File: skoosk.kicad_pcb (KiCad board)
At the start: 2 copper layers, 281.4 x 78.4 mm, 92 parts, among them SW1 SW_Push, U1 ProMicro

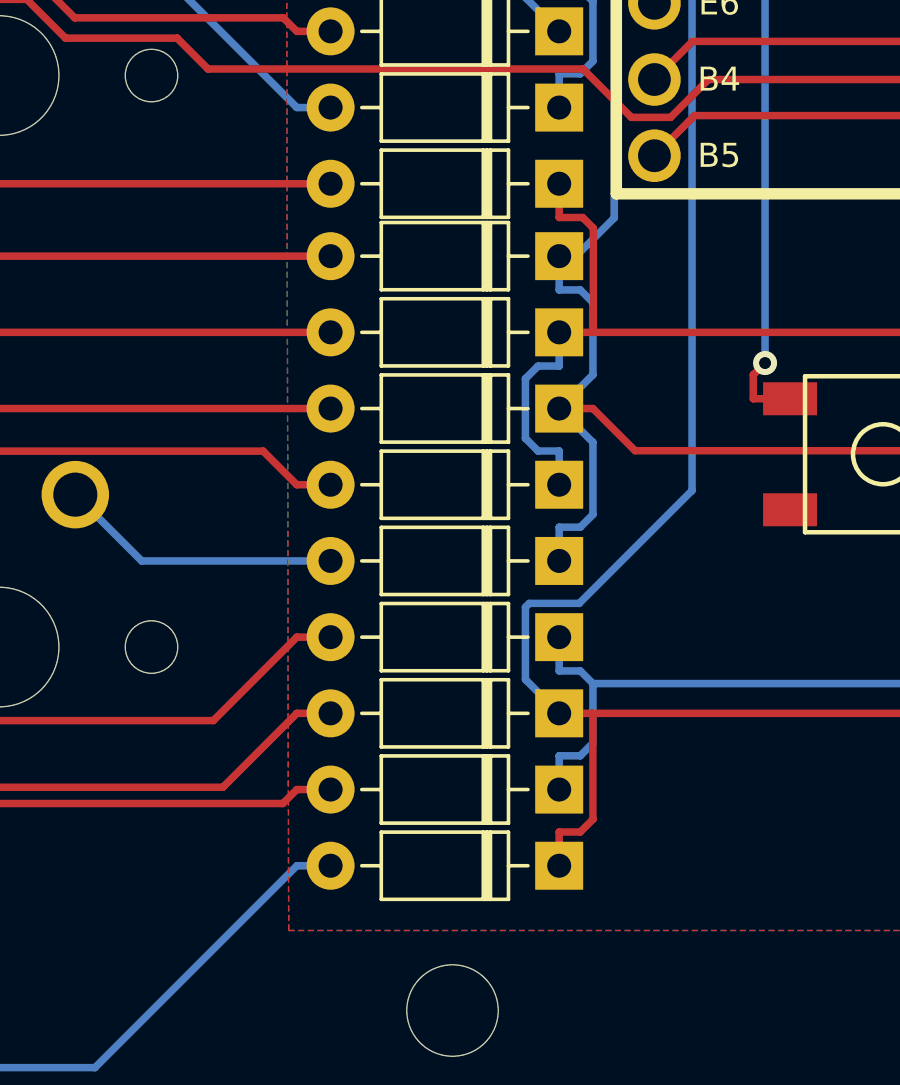
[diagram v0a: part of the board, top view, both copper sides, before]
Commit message: zero error return
add some led?
get feedback?
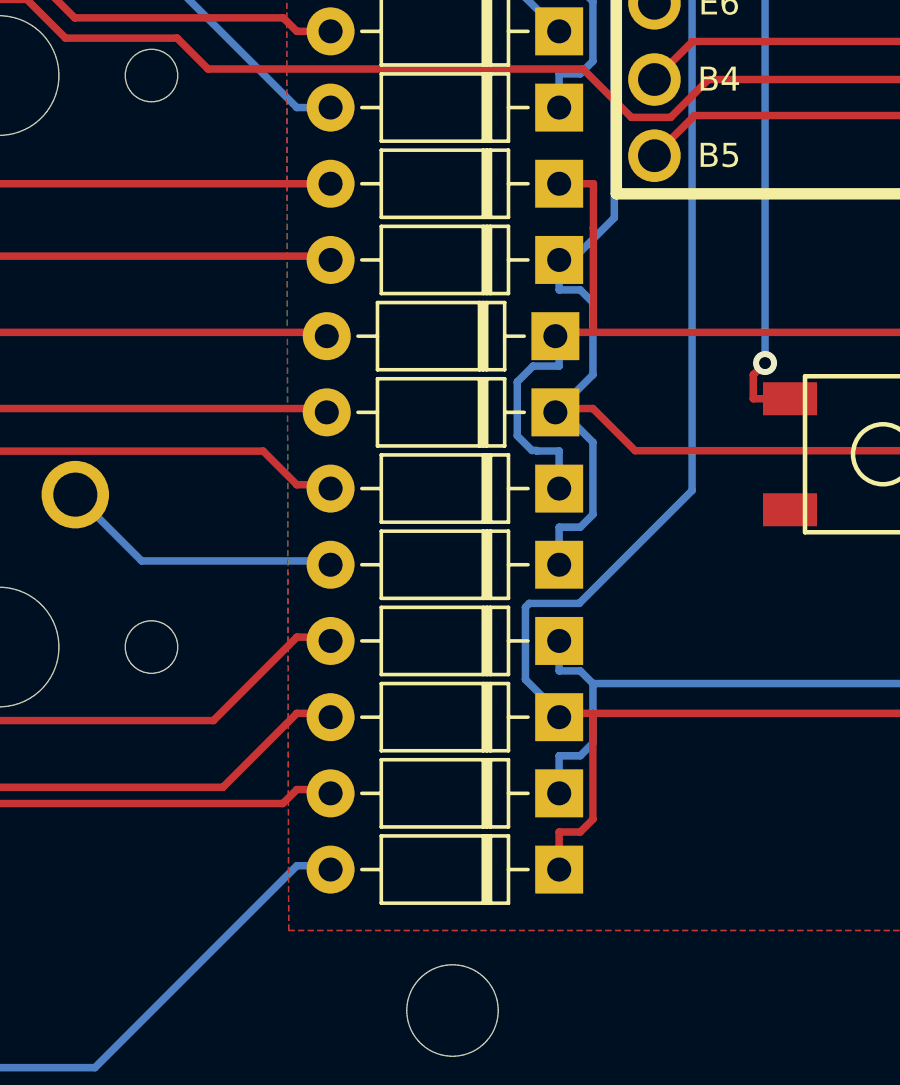
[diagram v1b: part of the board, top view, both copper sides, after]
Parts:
- moved D27 0.18 mm to (128.1, 49.1)
- moved D28 0.18 mm to (128.1, 51.7)
- moved D26 0.13 mm to (128.3, 46.6)
- moved D29 0.13 mm to (128.3, 54.2)
- moved D30 0.13 mm to (128.3, 56.8)
- moved D37 0.13 mm to (128.3, 59.3)
- moved D38 0.13 mm to (128.3, 61.8)
- moved D39 0.13 mm to (128.3, 64.4)
- moved D40 0.13 mm to (128.3, 66.9)
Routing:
- net ROW4: track 61.5 -> 62.1 mm
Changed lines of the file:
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@@
   (net 66 "unconnected-(U1-Pad1)")
   (footprint "Diode_THT:D_DO-35_SOD27_P7.62mm_Horizontal" (layer "F.Cu")
-    (at 128.27 51.562 180)
+    (at 128.143 51.689 180)
     (descr "Diode, DO-35_SOD27 series, Axial, Horizontal, pin pitch=7.62mm, , length*diameter=4*2mm^2, , http://www.diodes.com/_files/packages/DO-35.pdf")
     (tags "Diode DO-35_SOD27 series Axial Horizontal pin pitch 7.62mm  length 4mm diameter 2mm")
@@
   )
   (footprint "Diode_THT:D_DO-35_SOD27_P7.62mm_Horizontal" (layer "F.Cu")
-    (at 128.27 66.802 180)
+    (at 128.27 66.929 180)
     (descr "Diode, DO-35_SOD27 series, Axial, Horizontal, pin pitch=7.62mm, , length*diameter=4*2mm^2, , http://www.diodes.com/_files/packages/DO-35.pdf")
     (tags "Diode DO-35_SOD27 series Axial Horizontal pin pitch 7.62mm  length 4mm diameter 2mm")
@@
   )
   (footprint "Diode_THT:D_DO-35_SOD27_P7.62mm_Horizontal" (layer "F.Cu")
-    (at 128.27 64.262 180)
+    (at 128.27 64.389 180)
     (descr "Diode, DO-35_SOD27 series, Axial, Horizontal, pin pitch=7.62mm, , length*diameter=4*2mm^2, , http://www.diodes.com/_files/packages/DO-35.pdf")
     (tags "Diode DO-35_SOD27 series Axial Horizontal pin pitch 7.62mm  length 4mm diameter 2mm")
@@
   )
   (footprint "Diode_THT:D_DO-35_SOD27_P7.62mm_Horizontal" (layer "F.Cu")
-    (at 128.27 49.022 180)
+    (at 128.143 49.149 180)
     (descr "Diode, DO-35_SOD27 series, Axial, Horizontal, pin pitch=7.62mm, , length*diameter=4*2mm^2, , http://www.diodes.com/_files/packages/DO-35.pdf")
     (tags "Diode DO-35_SOD27 series Axial Horizontal pin pitch 7.62mm  length 4mm diameter 2mm")
@@
   )
   (footprint "Diode_THT:D_DO-35_SOD27_P7.62mm_Horizontal" (layer "F.Cu")
-    (at 128.27 56.642 180)
+    (at 128.27 56.769 180)
     (descr "Diode, DO-35_SOD27 series, Axial, Horizontal, pin pitch=7.62mm, , length*diameter=4*2mm^2, , http://www.diodes.com/_files/packages/DO-35.pdf")
     (tags "Diode DO-35_SOD27 series Axial Horizontal pin pitch 7.62mm  length 4mm diameter 2mm")
@@
   )
   (footprint "Diode_THT:D_DO-35_SOD27_P7.62mm_Horizontal" (layer "F.Cu")
-    (at 128.27 46.482 180)
+    (at 128.27 46.609 180)
     (descr "Diode, DO-35_SOD27 series, Axial, Horizontal, pin pitch=7.62mm, , length*diameter=4*2mm^2, , http://www.diodes.com/_files/packages/DO-35.pdf")
     (tags "Diode DO-35_SOD27 series Axial Horizontal pin pitch 7.62mm  length 4mm diameter 2mm")
@@
   )
   (footprint "Diode_THT:D_DO-35_SOD27_P7.62mm_Horizontal" (layer "F.Cu")
-    (at 128.27 54.102 180)
+    (at 128.27 54.229 180)
     (descr "Diode, DO-35_SOD27 series, Axial, Horizontal, pin pitch=7.62mm, , length*diameter=4*2mm^2, , http://www.diodes.com/_files/packages/DO-35.pdf")
     (tags "Diode DO-35_SOD27 series Axial Horizontal pin pitch 7.62mm  length 4mm diameter 2mm")
@@
   )
   (footprint "Diode_THT:D_DO-35_SOD27_P7.62mm_Horizontal" (layer "F.Cu")
-    (at 128.27 59.182 180)
+    (at 128.27 59.309 180)
     (descr "Diode, DO-35_SOD27 series, Axial, Horizontal, pin pitch=7.62mm, , length*diameter=4*2mm^2, , http://www.diodes.com/_files/packages/DO-35.pdf")
     (tags "Diode DO-35_SOD27 series Axial Horizontal pin pitch 7.62mm  length 4mm diameter 2mm")
@@
   )
   (footprint "Diode_THT:D_DO-35_SOD27_P7.62mm_Horizontal" (layer "F.Cu")
-    (at 128.27 61.722 180)
+    (at 128.27 61.849 180)
     (descr "Diode, DO-35_SOD27 series, Axial, Horizontal, pin pitch=7.62mm, , length*diameter=4*2mm^2, , http://www.diodes.com/_files/packages/DO-35.pdf")
     (tags "Diode DO-35_SOD27 series Axial Horizontal pin pitch 7.62mm  length 4mm diameter 2mm")
@@
   (segment (start 149.86 38.989) (end 149.86 37.8639) (width 0.25) (layer "B.Cu") (net 54))
   (segment (start 149.86 46.609) (end 148.7349 46.609) (width 0.25) (layer "F.Cu") (net 55))
+  (segment (start 128.27 44.069) (end 129.413 44.069) (width 0.25) (layer "F.Cu") (net 55))
   (segment (start 148.7349 46.609) (end 146.3219 49.022) (width 0.25) (layer "F.Cu") (net 55))
-  (segment (start 129.4088 45.5503) (end 129.0526 45.1941) (width 0.25) (layer "F.Cu") (net 55))
   (segment (start 129.4088 49.022) (end 129.4088 45.5503) (width 0.25) (layer "F.Cu") (net 55))
+  (segment (start 129.413 45.5461) (end 129.4088 45.5503) (width 0.25) (layer "F.Cu") (net 55))
   (segment (start 146.3219 49.022) (end 129.4088 49.022) (width 0.25) (layer "F.Cu") (net 55))
   (segment (start 149.86 51.689) (end 148.7349 51.689) (width 0.25) (layer "F.Cu") (net 55))
-  (segment (start 128.27 44.069) (end 128.27 45.1941) (width 0.25) (layer "F.Cu") (net 55))
-  (segment (start 129.0526 45.1941) (end 128.27 45.1941) (width 0.25) (layer "F.Cu") (net 55))
   (segment (start 129.4088 49.022) (end 128.27 49.022) (width 0.25) (layer "F.Cu") (net 55))
+  (segment (start 129.413 44.069) (end 129.413 45.5461) (width 0.25) (layer "F.Cu") (net 55))
   (segment (start 146.3219 49.022) (end 148.7349 51.435) (width 0.25) (layer "F.Cu") (net 55))
   (segment (start 148.7349 51.435) (end 148.7349 51.689) (width 0.25) (layer "F.Cu") (net 55))
-  (segment (start 128.27 54.102) (end 128.27 52.9769) (width 0.25) (layer "B.Cu") (net 55))
+  (segment (start 127.363 52.959) (end 126.873 52.469) (width 0.25) (layer "B.Cu") (net 55))
   (segment (start 150.9851 55.222) (end 150.5632 55.6439) (width 0.25) (layer "B.Cu") (net 55))
-  (segment (start 127.5668 52.9769) (end 127.1449 52.555) (width 0.25) (layer "B.Cu") (net 55))
+  (segment (start 127.508 52.959) (end 127.363 52.959) (width 0.25) (layer "B.Cu") (net 55))
   (segment (start 149.86 46.609) (end 148.0235 44.7725) (width 0.25) (layer "B.Cu") (net 55))
   (segment (start 148.0235 34.3132) (end 146.685 32.9747) (width 0.25) (layer "B.Cu") (net 55))
   (segment (start 150.5632 55.6439) (end 149.86 55.6439) (width 0.25) (layer "B.Cu") (net 55))
+  (segment (start 128.27 52.9769) (end 127.5259 52.9769) (width 0.25) (layer "B.Cu") (net 55))
   (segment (start 148.0235 44.7725) (end 148.0235 34.3132) (width 0.25) (layer "B.Cu") (net 55))
-  (segment (start 127.1449 52.555) (end 127.1449 50.569) (width 0.25) (layer "B.Cu") (net 55))
-  (segment (start 128.27 49.022) (end 128.27 50.1471) (width 0.25) (layer "B.Cu") (net 55))
+  (segment (start 128.27 54.102) (end 128.27 52.9769) (width 0.25) (layer "B.Cu") (net 55))
+  (segment (start 127.5259 52.9769) (end 127.508 52.959) (width 0.25) (layer "B.Cu") (net 55))
   (segment (start 149.86 56.769) (end 149.86 55.6439) (width 0.25) (layer "B.Cu") (net 55))
+  (segment (start 128.27 50.1471) (end 128.27 49.022) (width 0.25) (layer "B.Cu") (net 55))
   (segment (start 149.86 51.689) (end 150.9851 52.8141) (width 0.25) (layer "B.Cu") (net 55))
-  (segment (start 127.1449 50.569) (end 127.5668 50.1471) (width 0.25) (layer "B.Cu") (net 55))
-  (segment (start 128.27 52.9769) (end 127.5668 52.9769) (width 0.25) (layer "B.Cu") (net 55))
-  (segment (start 127.5668 50.1471) (end 128.27 50.1471) (width 0.25) (layer "B.Cu") (net 55))
+  (segment (start 127.3989 50.1471) (end 128.27 50.1471) (width 0.25) (layer "B.Cu") (net 55))
+  (segment (start 126.873 50.673) (end 127.3989 50.1471) (width 0.25) (layer "B.Cu") (net 55))
   (segment (start 150.9851 52.8141) (end 150.9851 55.222) (width 0.25) (layer "B.Cu") (net 55))
+  (segment (start 126.873 52.469) (end 126.873 50.673) (width 0.25) (layer "B.Cu") (net 55))
   (segment (start 128.27 51.562) (end 129.3951 51.562) (width 0.25) (layer "F.Cu") (net 56))
   (segment (start 149.86 54.229) (end 148.7349 54.229) (width 0.25) (layer "F.Cu") (net 56))
